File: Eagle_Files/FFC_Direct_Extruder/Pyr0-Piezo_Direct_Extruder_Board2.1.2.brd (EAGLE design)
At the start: 39.6 x 46.5 mm, 37 parts, among them J1 10118192-0001LF, U1 CP2102N-A01-GQFN28

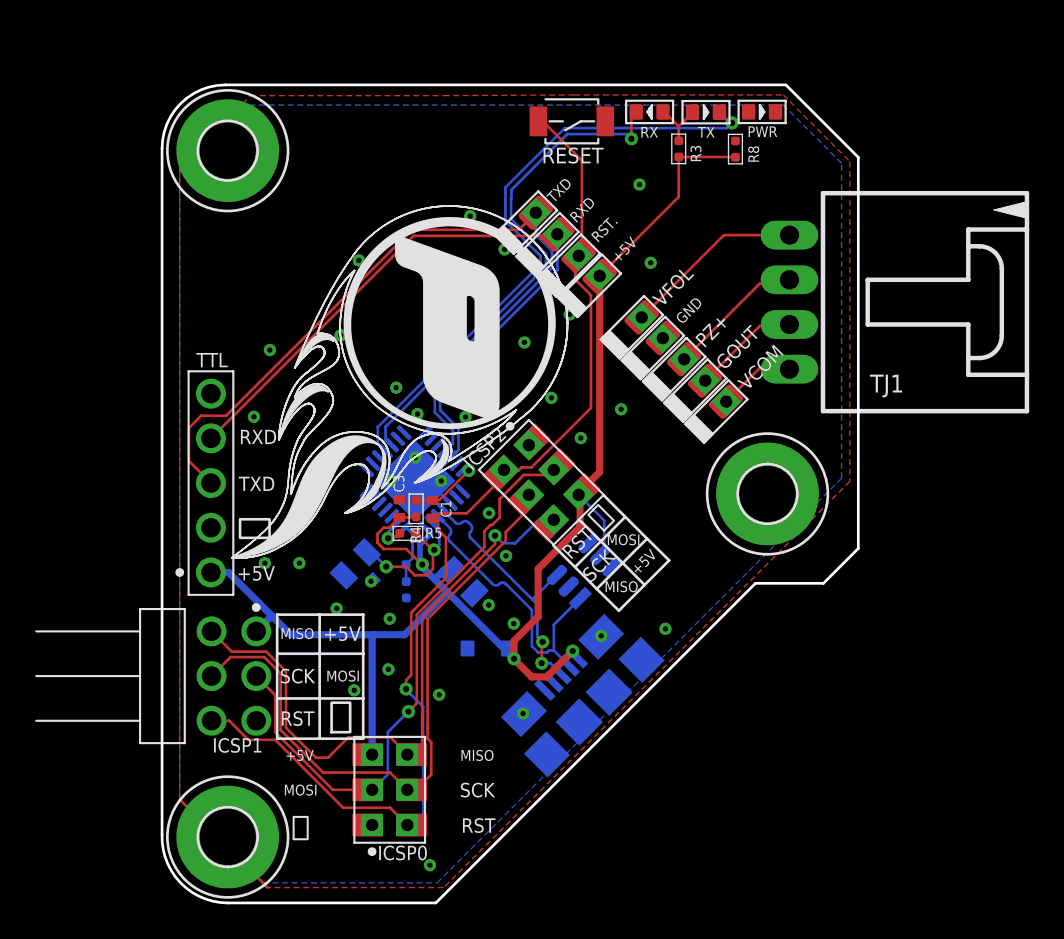
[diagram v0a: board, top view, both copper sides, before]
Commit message: Complete overhaul of FFC board for v2.1.2 #bugfix
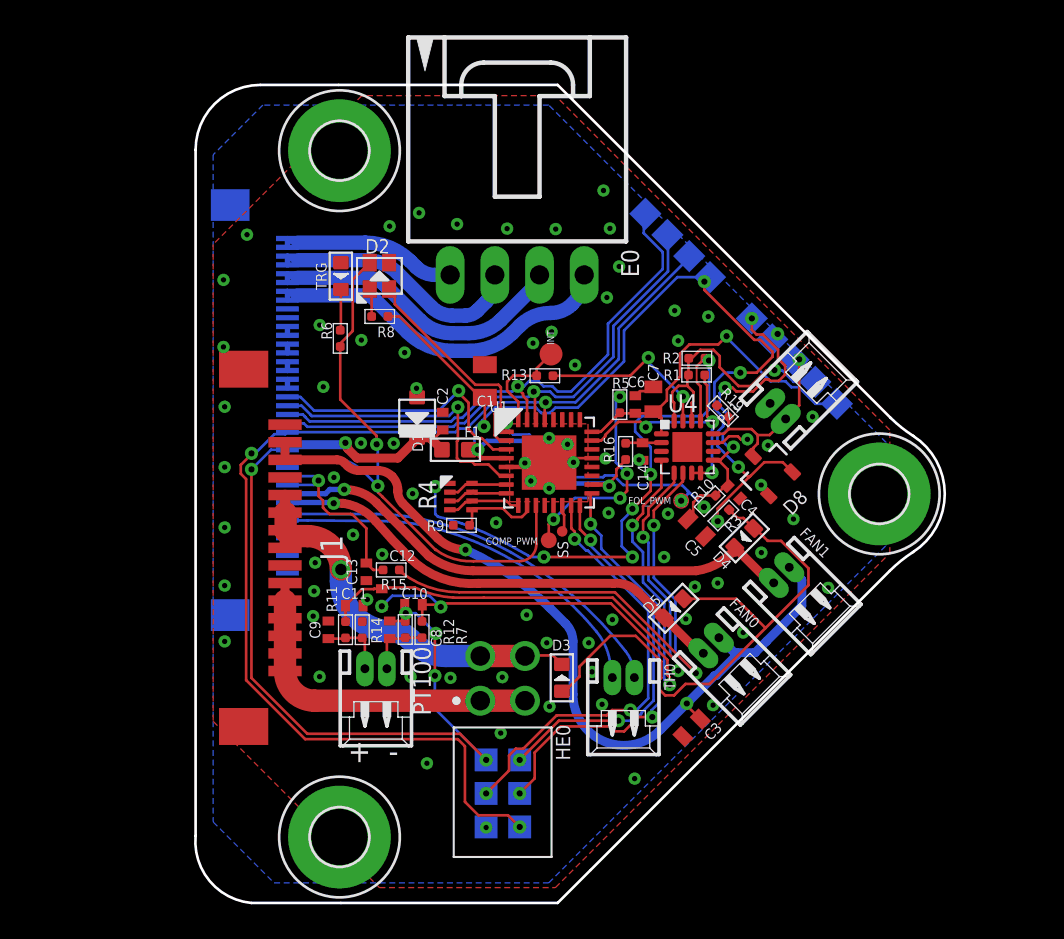
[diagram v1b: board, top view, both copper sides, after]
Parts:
- removed ICSP0, ICSP2: ICSP_HEADERSPRING_3.48X1.1, PiezoFFC:ICSP_3X2_3.48X1.1_SPRING_CONTACTS
- removed ICSP1: ICSP_HEADERICSP_2.54MM_RIGHT, PiezoFFC:ICSP_2X3_2.54_RIGHT
- removed PWR, RX, TX: (no value), PiezoFFC:SEEED-LED_LED-0603
- removed RESET: (no value), PiezoFFC:SEEED-SWITCH_SW2-2.6-3.0X2.5X1.2+0.4MM
- removed TJ1: C-GRID-04-70553, PiezoFFC:70553-04
- removed TTL: JST-2.54MM_5P-2.54JST_2.54MM_5P_F, PiezoFFC:HDRVR5W64P254_1X5_1270X254X575B
- removed VFOL: TPSPRING_CONTACT_3.5X1.1, PiezoFFC:SPRING_CONTACT_3.48X1.10
- added 5V, FOL, MISO, MOSI, RST, SCK: TPTP13SQ, PiezoFFC:TP13SQ
- added C10, C11, C14, C8, C9: 0.1uF, PiezoFFC:CAPC1005X50
- added C12: 1uF, PiezoFFC:CAPC1005X50
- added C13: 10nF, PiezoFFC:CAPC1005X50
- added C6: 10uF, PiezoFFC:CAPC1005X50
- added C7: 3.3uF, PiezoFFC:CAPC1609X80
- added COMP_PWM, FOL_PWM: TPTP09R, PiezoFFC:TP09R
- added D1: DIODE_ZENER_PLZ5V1C, PiezoFFC:DO-219AC
- added D4, D5, TRG: (no value), PiezoFFC:SEEED-LED_LED-0603
- added D8: BAV199, PiezoFFC:SOT23
- added E0: C-GRID-04-70553, PiezoFFC:70553-04
- added F1: 500mA, PiezoFFC:SEEED-RESISTOR_R0603
- added FAN0, FAN1, PT100, PZ1, TH0: CON-MOLEX-2P-1.27MM048, PiezoFFC:53048-02
- added HE0: JST-2.54-2X2JST-DUPONT-2.54-2X2, PiezoFFC:HDRRAR4W64P254_2X2_556X736X556B
- added INT: TPTP13R, PiezoFFC:TP13R
- added R10, R11, R7: 10K, PiezoFFC:R0402
- added R12, R14: 2K2, PiezoFFC:R0402
- added R13, R15, R16: 100R, PiezoFFC:R0402
- added R19: 1M, PiezoFFC:R0402
- added R6: 4K7, PiezoFFC:R0402
- added R9: 1K, PiezoFFC:R0402
- added SS: TPTP06R, testpad:TP06R
- added U4: LM2902QT, PiezoFFC:QFN16
- added X1: FFC-40P-0.5SH, PiezoFFC:FH12-40S-0.5SH
- added ⏚: TPTP13SQ, testpad:TP13SQ
- +5V, GND, RST., RXD, TXD: value TPSPRING_CONTACT_3.5X1.1 -> TPTP13SQ; device PiezoFFC:SPRING_CONTACT_3.48X1.10 -> testpad:TP13SQ
- C1: device PiezoFFC:CAPC1005X50 -> PiezoFFC:CAPC2012X130
- C3: value 0.1uF -> 1uF; device PiezoFFC:CAPC1005X50 -> PiezoFFC:CAPC1609X80
- C4: value 4.7uF -> 10uF; device PiezoFFC:CAPC2012X130 -> PiezoFFC:CAPC1005X50
- C5: value 4.7uF -> 3.3uF; device PiezoFFC:CAPC2012X130 -> PiezoFFC:CAPC1609X80
- D2: value DIODE_TVS_ARRAY_CM1293A -> LED-RGB-COM_ANO4PLCC; device PiezoFFC:SC-74-6 -> PiezoFFC:4PLCC
- D3: value DIODE_ZENER_PLZ5V1C -> (none); device PiezoFFC:DO-219AC -> PiezoFFC:SEEED-LED_LED-0603
- GOUT, PZ+, VCOM: value TPSPRING_CONTACT_3.5X1.1 -> TPTP13SQ; device PiezoFFC:SPRING_CONTACT_3.48X1.10 -> PiezoFFC:TP13SQ
- J1: value 10118192-0001LF -> FFC-15P-1MM; device PiezoFFC:AMPHENOL_10118192-0001LF -> PiezoFFC:FFC-15P-1MM
- R1: value 22K -> 1M
- R2: value 47K -> 10K
- R3: value (none) -> 2K2
- R4: value 10K -> 1K; device PiezoFFC:R0402 -> PiezoFFC:EXBN8V
- R5: value 10K -> 0R
- R8: value (none) -> 4K7
- U1: value CP2102N-A01-GQFN28 -> ATMEGA48/88/168/328PB; device PiezoFFC:QFN50P500X500X80-29N -> PiezoFFC:QFN50P500X500X90-33N
- moved R8 22.3 mm to (12.4, 33.5), turned to 270 degrees
- moved J1 21.1 mm to (6.99, 27.3), flipped to the top, turned to 270 degrees
- moved R2 21.1 mm to (30.4, 31.1), flipped to the top, turned to 270 degrees
- moved R3 21.0 mm to (31.9, 22.1), turned to 135 degrees
- moved C3 20.8 mm to (30.1, 10.1), turned to 225 degrees
- moved D2 20.4 mm to (12.3, 35.8), flipped to the top, turned to 90 degrees
- moved C5 19.5 mm to (30.4, 21.4), flipped to the top, turned to 135 degrees
- moved R1 19.3 mm to (30.4, 30.1), flipped to the top
- moved C4 16.2 mm to (32.5, 23.5), flipped to the top, turned to 135 degrees
- moved R5 14.1 mm to (26.0, 28.4), turned to 180 degrees
- moved U$1 9.60 mm to (22.6, 25.6), flipped to the bottom, turned to 0 degrees
- moved C2 9.34 mm to (15.9, 27.5), flipped to the top, turned to 270 degrees
- moved VCOM 9.04 mm to (38.3, 28.5), flipped to the bottom, turned to 45 degrees
- moved C1 7.87 mm to (18.3, 29.8)
- moved U1 7.69 mm to (22.0, 25.1), flipped to the top, turned to 0 degrees
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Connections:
- removed net 5V_DC: +5V.TH, +5V.TP, C3.2, C4.1, D2.5, D3.P$2, ICSP0.5, ICSP0.P$5, ICSP1.1, ICSP2.5, ICSP2.P$5, J1.1, R1.2, R3.1, R4.1, R8.1, TTL.1, TTL.5, U1.7
- removed net D+: D2.3, J1.3, U1.4
- removed net D-: D2.1, J1.2, U1.5
- removed net GOUT: GOUT.TH, GOUT.TP, TJ1.3
- removed net PGM_RST: C1.2, R4.2, U1.28
- removed net PWR_IND: PWR.+, R8.2
- removed net RST_PULLUP: R5.1, U1.9
- removed net RXD: RXD.TH, RXD.TP, TTL.4, U1.26
- removed net RXT: RX.-, U1.19
- removed net TXD: TTL.3, TXD.TH, TXD.TP, U1.25
- removed net TXT: TX.-, U1.18
- removed net VBUS: R1.1, R2.2, U1.8
- removed net VCOM: PZ+.TH, PZ+.TP, TJ1.4
- removed net VDD: C2.2, C5.1, R5.2, U1.6
- removed net VFOL: TJ1.1, VFOL.TH, VFOL.TP
- new net +5V: +5V.TP, C1.1, D8.2, F1.2, R16.2, R3.1, R8.1, U1.18, U1.4
- new net COMP_VCC: C14.2, R16.1, U4.2
- new net E0_1A: E0.2, X1.37, X1.38
- new net E0_1B: E0.1, X1.39, X1.40
- new net E0_2A: E0.3, X1.35, X1.36
- new net E0_2B: E0.4, X1.33, X1.34
- new net ERR_LED: D2.P$2, U1.2
- new net FAN0_GATE: D5.-, FAN0.1, X1.10
- new net FAN1_GATE: D4.-, FAN1.1, X1.11
- new net GADJ_R0: R4.2, R4.8, U1.7
- new net GADJ_R1: R4.3, R4.7, U1.8
- new net GADJ_R2: R4.4, R4.6, U1.9
- new net GADJ_R3: R4.5, R9.2, U1.10
- new net GAIN_FB: R2.1, R4.1, U4.13
- new net GAIN_OUT: GOUT.TP, R1.2, R2.2, U4.14, U4.16
- new net HE0-: D3.-, HE0.3, HE0.4, J1.P$5, J1.P$6, J1.P$7, J1.P$8
- new net PT100+: C8.1, PT100.2, R12.1, R7.2
- new net PT100-: C9.2, PT100.1, R11.2, R14.2
- new net PT100_AMP+: C10.1, C12.2, R7.1, U4.4
- new net PT100_AMP-: C11.2, C12.1, R11.1, U4.5
- new net PT100_OUT: C13.2, R15.1, X1.12, X1.13
- new net PT100_R: R15.2, U4.6
- new net PZ_AMP_OUT: R13.1, U4.15
- new net RGB_VCC: D2.P$1, R8.2
- new net SCL: U1.6, X1.21
- new net SDA: U1.3, X1.22
- new net SPI_SS: SS.TP, U1.14
- new net TH0+: TH0.1, X1.8
- new net TH0-: TH0.2, X1.9
- new net TRG_LED: R6.2, TRG.-
- new net TTL_RXD: RXD.TP, U1.30, X1.19
- new net TTL_TXD: TXD.TP, U1.31, X1.20
- new net VCC: HE0.1, HE0.2, J1.P$10, J1.P$11, J1.P$12, J1.P$13, J1.P$14, J1.P$15
- new net VCC_REG: 5V.TP, C10.2, C2.2, C8.2, D1.P$2, F1.1, R12.2, X1.16, X1.17
- new net VCOMP_PWM: COMP_PWM.TP, R5.2, U1.13
- new net VCOMP_SENSE: C6.2, C7.2, R5.1, U1.24, U4.1, VCOM.TP
- new net VREF_IN: C4.2, C5.2, FOL.TP, R10.1, U4.9
- new net V_FOLLOW: R1.1, U1.23, U4.7, U4.8
- new net V_FOL_PWM: FOL_PWM.TP, R10.2, U1.1
- new net V_INT: C3.1, FAN0.2, FAN1.2, J1.P$2, J1.P$3
- new net X_1A: X1.27, X1.28
- new net X_1B: X1.29, X1.30
- new net X_2A: X1.25, X1.26
- new net X_2B: X1.23, X1.24
- new net X_MIN_TRIG: X1.14
- new net Z_MIN_TRIG: D2.P$4, R6.1, U1.11, X1.15
- new net Z_TRG: INT.TP, R13.2, U1.32
- net GND: now also C1.2, C11.1, C13.1, C14.1, C3.2, C4.1, C5.1, C6.1, C7.1, C9.1, D1.P$1, D2.P$3, D8.1, J1.P$1, J1.P$16, J1.P$17, J1.P$4, J1.P$9, PZ1.2, R14.1, R19.1, R9.1, TRG.+, U1.21, U1.33, U1.5, U4.11, X1.1, X1.2, X1.3, X1.31, X1.32, X1.4, X1.5, X1.6, X1.7, ⏚.TP; no longer C3.1, C4.2, C5.2, D2.2, D3.P$1, GND.TH, ICSP0.1, ICSP0.P$1, ICSP1.3, ICSP2.1, ICSP2.P$1, J1.5, J1.SH1, J1.SH2, J1.SH3, J1.SH4, J1.SH5, J1.SH6, PWR.-, R2.1, RESET.1, TTL.2, U1.29, U1.3
- net LED_VCC: now also D3.+, D4.+, D5.+; no longer RX.+, TX.+
- net PZ+: now also D8.3, PZ+.TP, PZ1.1, R19.2, U4.12; no longer TJ1.2, VCOM.TH, VCOM.TP
- net RST: now also RST.TP, U1.29, X1.18; no longer C1.1, ICSP0.2, ICSP0.P$2, ICSP1.4, ICSP2.2, ICSP2.P$2, RESET.2, RST..TH
- net SPI_MISO: now also MISO.TP, U1.16; no longer ICSP0.6, ICSP0.P$6, ICSP1.6, ICSP2.6, ICSP2.P$6
- net SPI_MOSI: now also MOSI.TP, U1.15; no longer ICSP0.4, ICSP0.P$4, ICSP1.2, ICSP2.4, ICSP2.P$4
- net SPI_SCK: now also SCK.TP, U1.17; no longer ICSP0.3, ICSP0.P$3, ICSP1.5, ICSP2.3, ICSP2.P$3
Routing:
- net 5V_DC: track 88.1 -> 0.00 mm, vias 3 -> 0
- net +5V: track 0.00 -> 66.1 mm, vias 0 -> 7
- net VCC_REG: track 0.00 -> 53.8 mm, vias 0 -> 6
- net V_INT: track 0.00 -> 46.1 mm, vias 0 -> 2
- net TXD: track 45.8 -> 0.00 mm
- net RXD: track 40.6 -> 0.00 mm
- net PT100_AMP+: track 0.00 -> 36.0 mm, vias 0 -> 4
- net TXT: track 35.2 -> 0.00 mm, vias 1 -> 0
- net PT100_AMP-: track 0.00 -> 35.1 mm, vias 0 -> 2
- net GAIN_FB: track 0.00 -> 34.6 mm, vias 0 -> 6
- net Z_MIN_TRIG: track 0.00 -> 33.3 mm, vias 0 -> 2
- net TTL_TXD: track 0.00 -> 32.3 mm, vias 0 -> 1
- net PT100_R: track 0.00 -> 32.1 mm, vias 0 -> 2
- net FAN1_GATE: track 0.00 -> 30.6 mm, vias 0 -> 1
- net TTL_RXD: track 0.00 -> 30.4 mm, vias 0 -> 1
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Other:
- board size 39.6 x 46.5 mm -> 42.6 x 46.5 mm
- board text added: "+ -"
- board text added: "2B 2A 1A 1B"
- board text added: "Fan0"
- board text added: "Fan1"
- board text added: "HE0"
- board text added: "PZ1"
- board text added: "TH0"
- board text removed: "+5V"
- board text removed: "GOUT"
- board text removed: "MISO"
- board text removed: "MOSI"
- board text removed: "PZ+"
- board text removed: "RST"
- board text removed: "RXD"
- board text removed: "SCK"
- board text removed: "TXD"
- board text removed: "VCOM"
- board text removed: "VFOL"
- board text removed: "⏚"
